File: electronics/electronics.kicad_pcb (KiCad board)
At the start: 2 copper layers, 62.9 x 38.8 mm, 14 parts, among them U1 ESP32-S3-WROOM-1, U3 NCP1117-3.3_SOT223, U4 U4, U5 NCP1117-3.3_SOT223

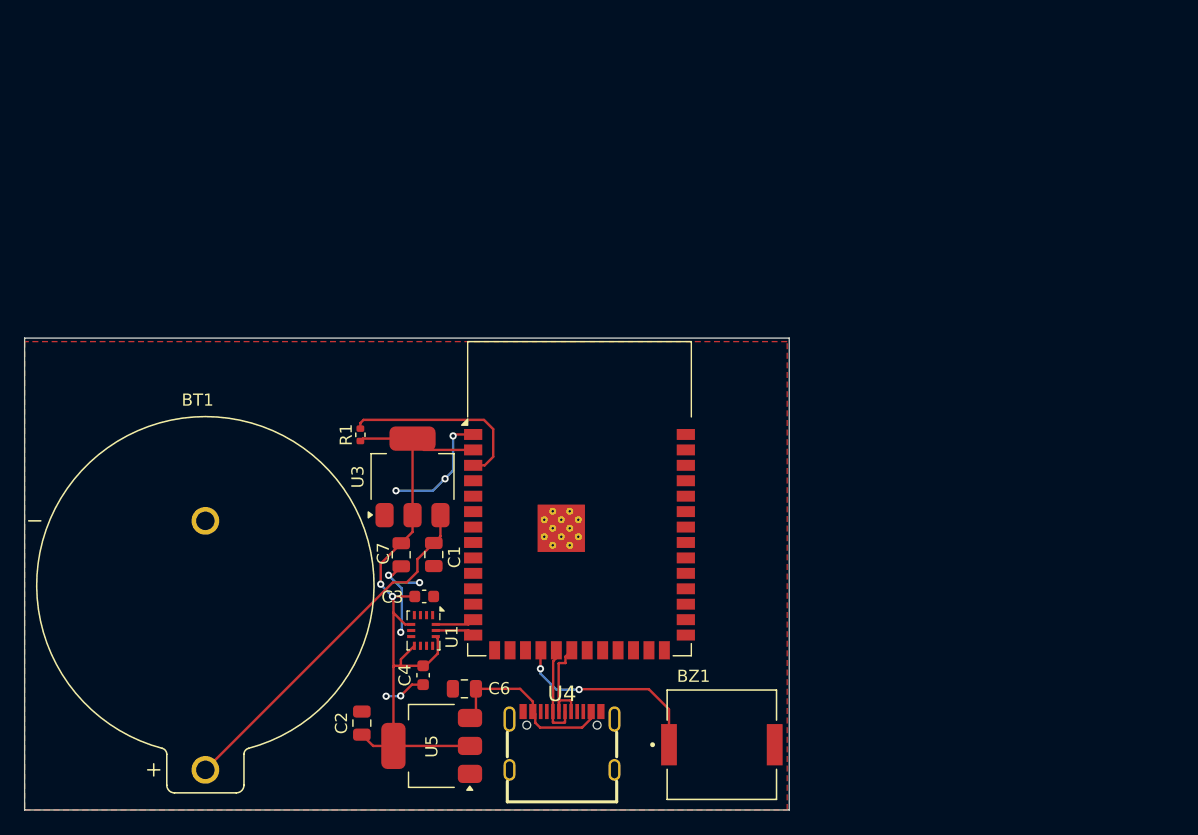
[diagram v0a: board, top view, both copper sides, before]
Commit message: BOM + Gerbers: Final Iteration (Hopefully)
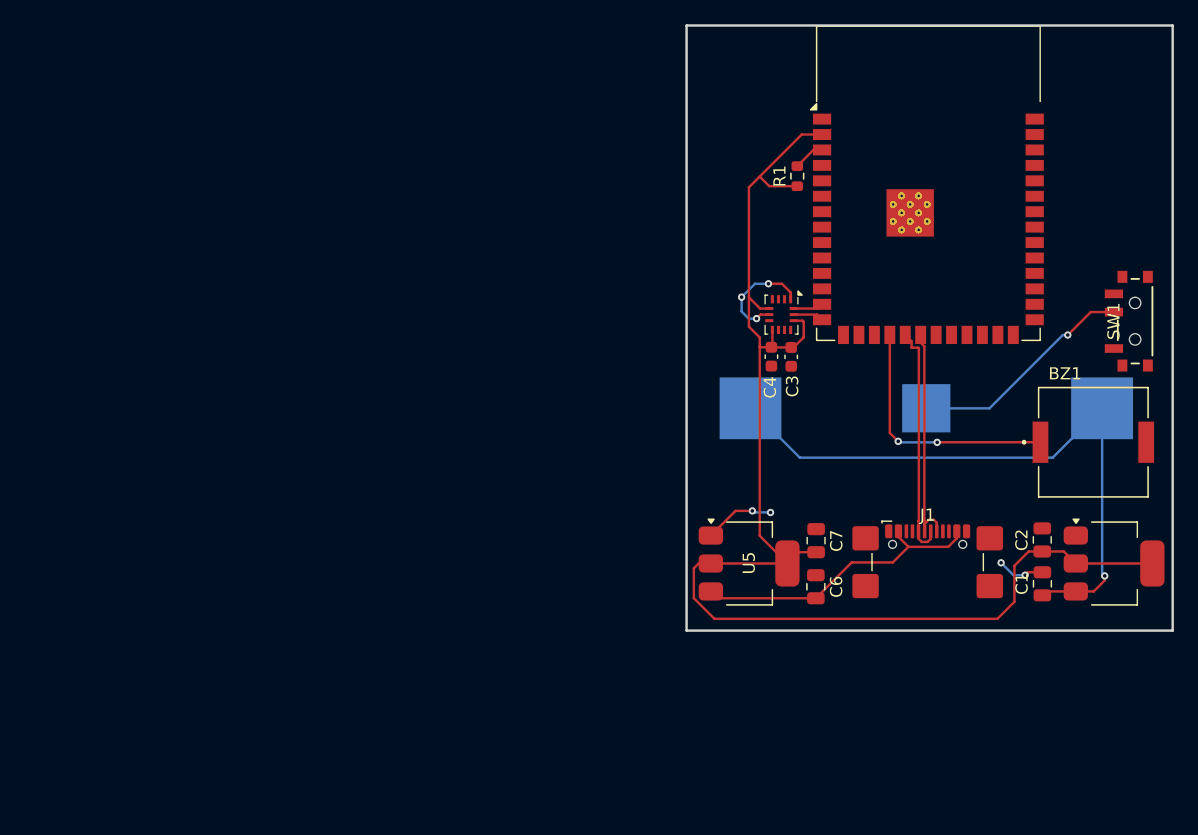
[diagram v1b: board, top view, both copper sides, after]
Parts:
- removed U4: U4, Uni:USB-C-SMD_G-SWITCH_GT-USB-7010ASV
- added J1: USB_C_Receptacle_USB2.0_14P, Connector_USB:USB_C_Receptacle_GCT_USB4110, F.Cu at (204.9, 105.3)
- added SW1: SW_SPDT, Uni:CUS-12TB_NDC, F.Cu at (222.0, 84.3)
- BT1: footprint Uni:BAT_1025 -> Uni:BAT_3024-2; moved to B.Cu
- R1: footprint Resistor_SMD:R_0402_1005Metric -> Resistor_SMD:R_0603_1608Metric
- moved BT1 61.1 mm to (204.8, 91.5), turned to 180 degrees
- moved U3 58.2 mm to (220.3, 104.3), turned to 0 degrees
- moved C2 58.0 mm to (214.4, 102.3)
- moved C1 50.1 mm to (214.4, 106.0), turned to 90 degrees
- moved R1 41.8 mm to (194.2, 72.4)
- moved BZ1 39.4 mm to (218.6, 94.3)
- moved U2 39.3 mm to (192.9, 83.8)
- moved C4 38.8 mm to (192.1, 87.3)
- moved U1 38.7 mm to (205.0, 73.0)
- moved C3 36.1 mm to (193.7, 87.3), turned to -90 degrees
- moved C7 34.2 mm to (195.8, 102.4), turned to 90 degrees
- moved U5 30.1 mm to (190.2, 104.3), turned to 0 degrees
- moved C6 30.1 mm to (195.7, 106.2), turned to 90 degrees
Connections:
- BT1 pad 2: GND -> Net-(BT1--)
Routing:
- net +3V3: track 57.2 -> 109.1 mm, vias 2 -> 0
- net Net-(BT1-+): track 29.7 -> 52.2 mm, vias 0 -> 1
- net Net-(BT1--): track 0.00 -> 18.9 mm, vias 0 -> 1
- net Net-(U1-EN): track 16.0 -> 2.59 mm
- net /D-: track 7.94 -> 19.4 mm
- net /D+: track 8.59 -> 18.9 mm
- net Net-(U5-VI): track 15.2 -> 24.7 mm
- net /BZR: track 16.7 -> 20.8 mm
- net GND: track 21.9 -> 18.9 mm, vias 8 -> 7
- net /SDA: track 3.24 -> 2.47 mm
- net /SCL: track 3.23 -> 2.50 mm
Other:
- board size 62.9 x 38.8 mm -> 40 x 49.8 mm
